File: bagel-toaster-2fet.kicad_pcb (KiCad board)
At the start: 2 copper layers, 142.6 x 62.6 mm, 118 parts, among them J1 bx, J10 9v, J11 9v, J12 9v, J13 9v, J14 o1b, J15 gnd, J16 gnd, J17 gnd, J18 gnd, J19 i2b, J2 do_snd, J20 o2b, J21 i2, J22 i2s, J23 gnd, J24 o2, J25 9v, J26 o2s, J27 i1, J28 i1s, J29 gnd, J3 out, J30 o1, J31 9v, J32 o1s, J4 in, J5 do_rtn, J6 i1b, J7 bs, J8 gnd, J9 9v, Q1 J113, Q2 J201, SW1 3pdt, SW2 Alpha_3PDT, SW3 Alpha_3PDT, SW4 Alpha_3PDT, U1 TL074, U2 4069

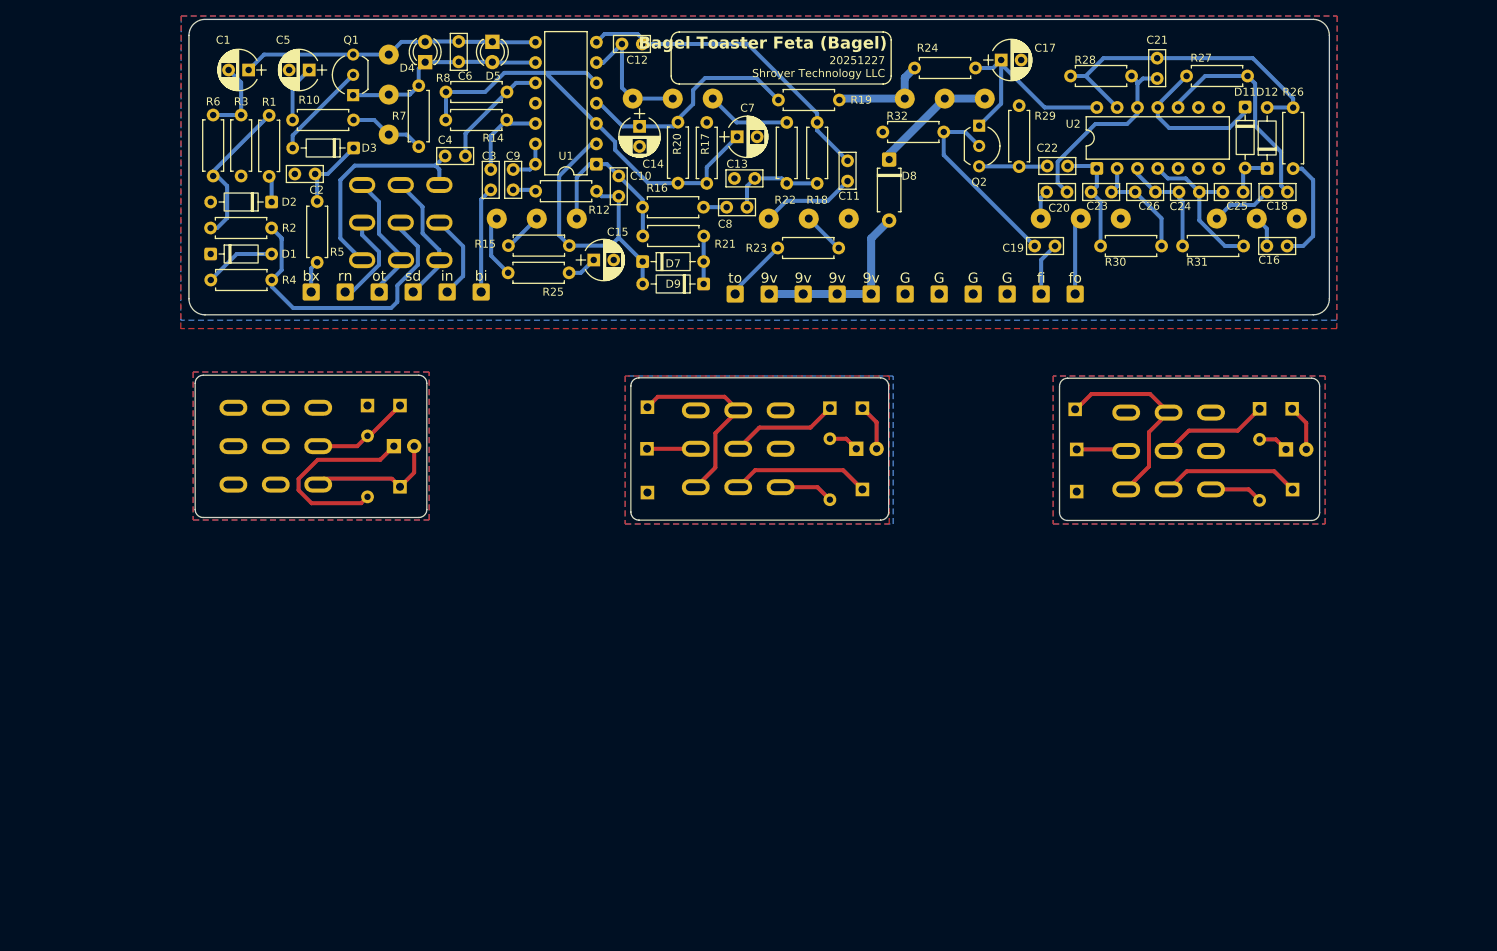
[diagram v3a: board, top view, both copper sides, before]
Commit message: 1590dd
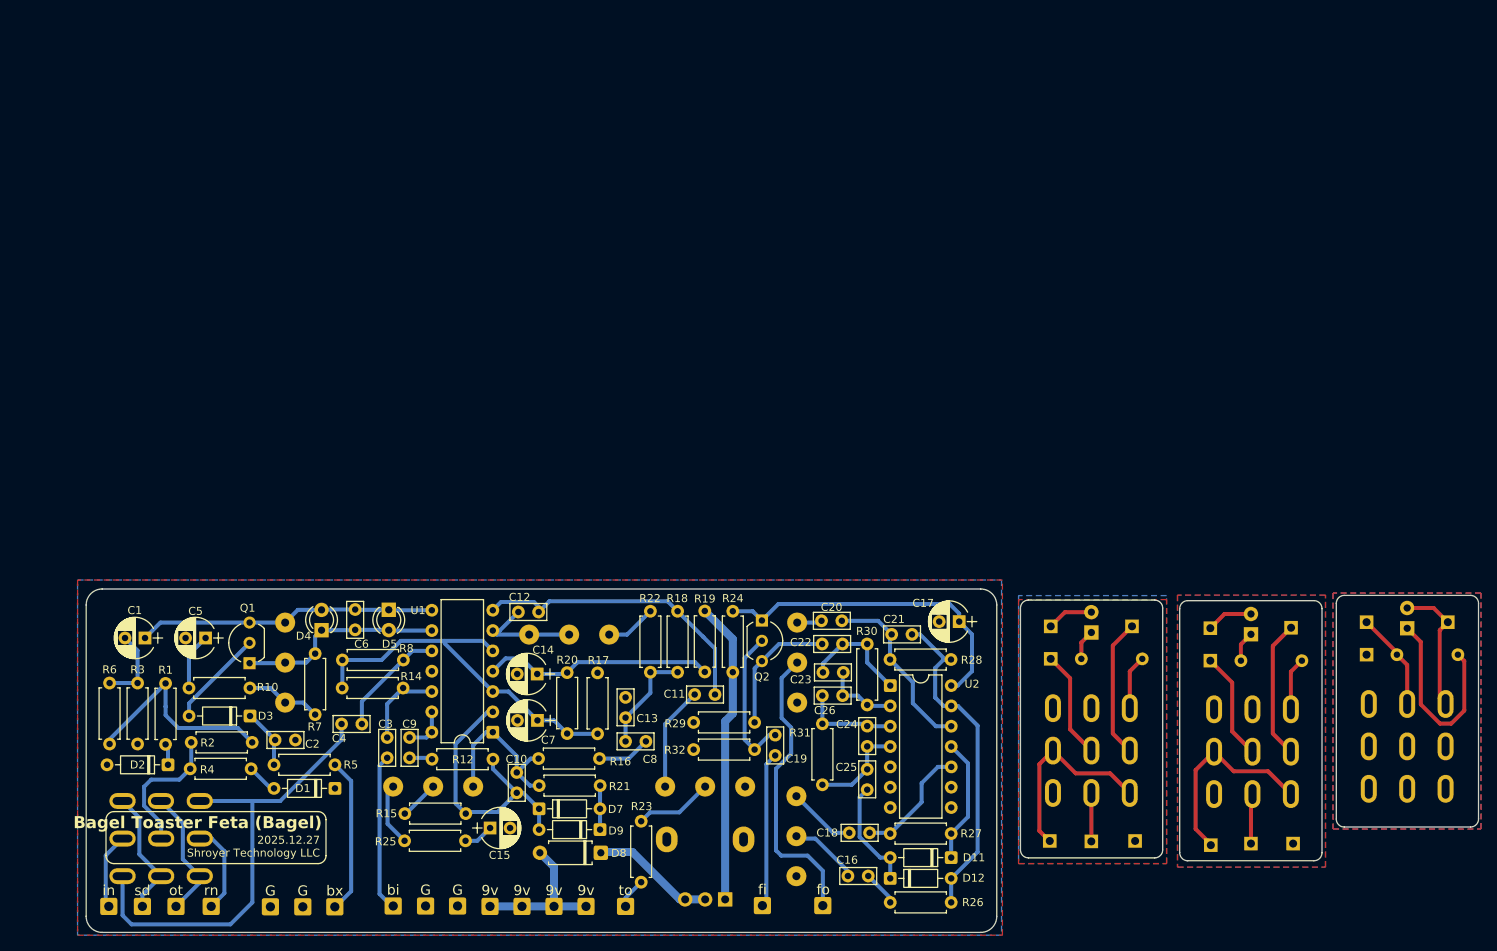
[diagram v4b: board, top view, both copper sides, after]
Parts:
- J14: value o1b -> to
- J19: value i2b -> fi
- J20: value o2b -> fo
- J6: value i1b -> bi
- J7: value bs -> bx
- sag1: footprint 1_mylib-footprint:pot-16mm-short-leg -> Potentiometer_THT:Potentiometer_Alpha_RD901F-40-00D_Single_Vertical
- moved SW2 146.3 mm to (216.8, 117.8), turned to -90 degrees
- moved J9 132.1 mm to (221.8, 102.3), turned to 90 degrees
- moved R13 131.6 mm to (215.5, 106.3), turned to 0 degrees
- moved J8 128.7 mm to (211.7, 106.3), turned to -90 degrees
- moved D6 128.7 mm to (216.8, 103.0), turned to 90 degrees
- moved J7 123.8 mm to (211.7, 102.3), turned to -90 degrees
- moved J17 119.8 mm to (74.7, 137.8)
- moved J16 110.4 mm to (78.7, 137.8)
- moved R26 104.6 mm to (152.1, 137.3), turned to 0 degrees
- moved J18 102.7 mm to (94.0, 137.8)
- moved splat1 101.8 mm to (155.9, 129.0), turned to 90 degrees
- moved D11 100.8 mm to (159.8, 131.7), turned to 180 degrees
- moved D12 100.5 mm to (152.1, 134.3), turned to 0 degrees
- moved R27 99.2 mm to (159.8, 128.7), turned to 180 degrees
- moved C18 95.6 mm to (149.6, 128.6)
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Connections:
- net /sg1 renamed Net-(J29-Pin_1)
- net /sg2 renamed Net-(J23-Pin_1)
- net /sg3 renamed Net-(J8-Pin_1)
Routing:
- net /b_snd: track 28.1 -> 58.0 mm
- net Net-(J20-Pin_1): track 9.72 -> 36.8 mm
- net Net-(R19-Pad1): track 12.6 -> 37.9 mm
- net /b_rtn: track 37.3 -> 17.4 mm
- net Net-(J1-Pin_1): track 4.02 -> 19.5 mm
- net /v1: track 27.7 -> 41.3 mm
- net Net-(J19-Pin_1): track 6.72 -> 19.4 mm
- net Net-(C18-Pad1): track 27.2 -> 15.1 mm
- net /vref: track 57.5 -> 47.9 mm
- net Net-(C16-Pad1): track 13.9 -> 4.44 mm
- net Net-(D11-A): track 5.88 -> 13.8 mm
- net Net-(Q2-S): track 8.57 -> 16.5 mm
- net Net-(C24-Pad2): track 19.7 -> 12.2 mm
- net Net-(R1-Pad1): track 19.3 -> 26.7 mm
- net Net-(J6-Pin_1): track 13.3 -> 19.5 mm
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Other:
- board size 142.6 x 62.6 mm -> 174 x 42.9 mm
- board text added: "2025.12.27 Shroyer Technology LLC"
- board text removed: "20251227 Shroyer Technology LLC"
